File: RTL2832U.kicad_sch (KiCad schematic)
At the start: 47 parts, among them U5 RTL2832U, U6 M24C02-WMN

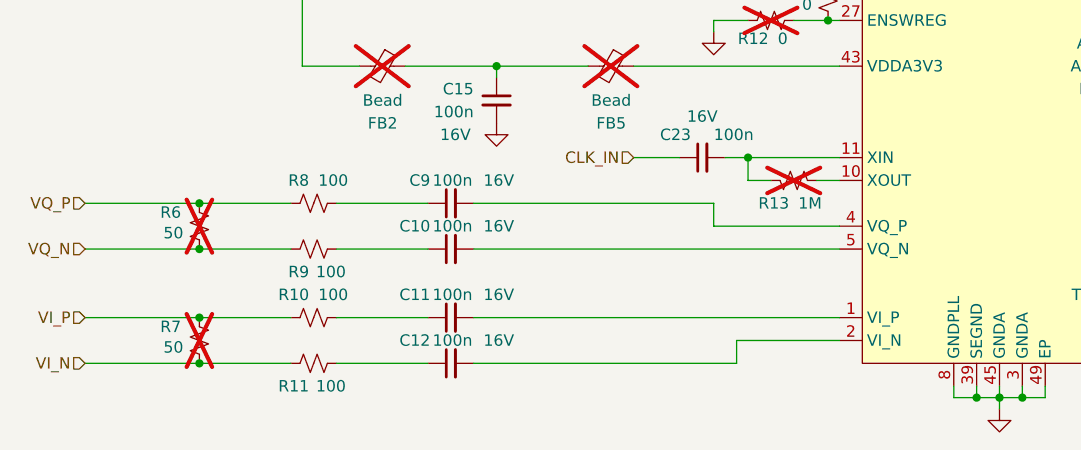
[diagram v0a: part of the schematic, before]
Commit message: PCB Layout Progress
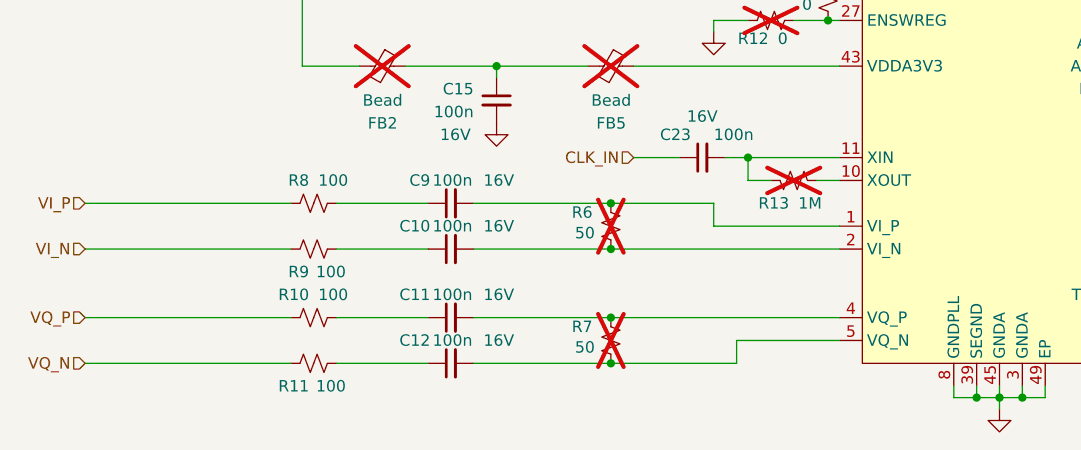
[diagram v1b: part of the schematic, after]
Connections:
- net VI_N: now also R9.2; no longer R11.2, R7.1
- net VI_P: now also R8.1; no longer R10.1, R7.2
- net VQ_N: now also R11.2; no longer R6.1, R9.2
- net VQ_P: now also R10.1; no longer R6.2, R8.1
- net at C11.2: now also R7.2, U5.4 (VQ_P); no longer U5.1 (VI_P)
- net at C10.2: now also R6.1, U5.2 (VI_N); no longer U5.5 (VQ_N)
- net at C12.2: now also R7.1, U5.5 (VQ_N); no longer U5.2 (VI_N)
- net at C9.2: now also R6.2, U5.1 (VI_P); no longer U5.4 (VQ_P)
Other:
- moved on the sheet: R6, R7
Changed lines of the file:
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@@
 	)
 	(junction
+		(at 143.51 195.58)
+		(diameter 0)
+		(color 0 0 0 0)
+	)
+	(junction
 		(at 167.64 152.4)
 		(diameter 0)
@@
 	)
 	(junction
-		(at 97.79 182.88)
-		(diameter 0)
-		(color 0 0 0 0)
-	)
-	(junction
 		(at 236.22 139.7)
 		(diameter 0)
@@
 	)
 	(junction
+		(at 143.51 182.88)
+		(diameter 0)
+		(color 0 0 0 0)
+	)
+	(junction
 		(at 184.15 204.47)
 		(diameter 0)
@@
 	)
 	(junction
+		(at 143.51 200.66)
+		(diameter 0)
+		(color 0 0 0 0)
+	)
+	(junction
 		(at 138.43 106.68)
 		(diameter 0)
@@
 	)
 	(junction
-		(at 97.79 187.96)
+		(at 231.14 144.78)
 		(diameter 0)
 		(color 0 0 0 0)
 	)
 	(junction
-		(at 231.14 144.78)
+		(at 143.51 187.96)
 		(diameter 0)
 		(color 0 0 0 0)
@@
 	)
 	(junction
-		(at 97.79 200.66)
-		(diameter 0)
-		(color 0 0 0 0)
-	)
-	(junction
 		(at 105.41 124.46)
 		(diameter 0)
@@
 	)
 	(junction
-		(at 97.79 195.58)
-		(diameter 0)
-		(color 0 0 0 0)
-	)
-	(junction
 		(at 167.64 119.38)
 		(diameter 0)
@@
 	(wire
 		(pts
-			(xy 85.09 187.96) (xy 97.79 187.96)
+			(xy 85.09 187.96) (xy 107.95 187.96)
 		)
 		(stroke
@@
 	(wire
 		(pts
-			(xy 128.27 195.58) (xy 168.91 195.58)
+			(xy 128.27 195.58) (xy 143.51 195.58)
 		)
 		(stroke
@@
 	(wire
 		(pts
+			(xy 143.51 200.66) (xy 157.48 200.66)
+		)
+		(stroke
+			(width 0)
+			(type default)
+		)
+	)
+	(wire
+		(pts
 			(xy 231.14 160.02) (xy 231.14 144.78)
 		)
@@
 	(wire
 		(pts
-			(xy 85.09 200.66) (xy 97.79 200.66)
+			(xy 85.09 200.66) (xy 107.95 200.66)
 		)
 		(stroke
@@
 	(wire
 		(pts
-			(xy 97.79 182.88) (xy 107.95 182.88)
-		)
-		(stroke
-			(width 0)
-			(type default)
-		)
-	)
-	(wire
-		(pts
-			(xy 85.09 195.58) (xy 97.79 195.58)
+			(xy 85.09 195.58) (xy 107.95 195.58)
 		)
 		(stroke
@@
 	(wire
 		(pts
-			(xy 128.27 200.66) (xy 157.48 200.66)
+			(xy 128.27 200.66) (xy 143.51 200.66)
 		)
 		(stroke
@@
 	(wire
 		(pts
+			(xy 143.51 195.58) (xy 168.91 195.58)
+		)
+		(stroke
+			(width 0)
+			(type default)
+		)
+	)
+	(wire
+		(pts
 			(xy 236.22 139.7) (xy 246.38 139.7)
 		)
@@
 	(wire
 		(pts
-			(xy 97.79 195.58) (xy 107.95 195.58)
-		)
-		(stroke
-			(width 0)
-			(type default)
-		)
-	)
-	(wire
-		(pts
 			(xy 229.87 88.9) (xy 229.87 91.44)
 		)
@@
 	(wire
 		(pts
-			(xy 85.09 182.88) (xy 97.79 182.88)
+			(xy 85.09 182.88) (xy 107.95 182.88)
+		)
+		(stroke
+			(width 0)
+			(type default)
+		)
+	)
+	(wire
+		(pts
+			(xy 143.51 182.88) (xy 154.94 182.88)
 		)
 		(stroke
@@
 	(wire
 		(pts
-			(xy 97.79 200.66) (xy 107.95 200.66)
-		)
-		(stroke
-			(width 0)
-			(type default)
-		)
-	)
-	(wire
-		(pts
 			(xy 223.52 152.4) (xy 246.38 152.4)
 		)
@@
 	(wire
 		(pts
-			(xy 97.79 187.96) (xy 107.95 187.96)
+			(xy 143.51 187.96) (xy 168.91 187.96)
 		)
 		(stroke
@@
 	(wire
 		(pts
-			(xy 128.27 187.96) (xy 168.91 187.96)
+			(xy 128.27 187.96) (xy 143.51 187.96)
 		)
 		(stroke
@@
 	(wire
 		(pts
-			(xy 128.27 182.88) (xy 154.94 182.88)
+			(xy 128.27 182.88) (xy 143.51 182.88)
 		)
 		(stroke
@@
 	(hierarchical_label "VI_N"
 		(shape input)
-		(at 85.09 200.66 180)
+		(at 85.09 187.96 180)
 		(effects
 			(font
@@
 	(hierarchical_label "VQ_P"
 		(shape input)
-		(at 85.09 182.88 180)
+		(at 85.09 195.58 180)
 		(effects
 			(font
@@
 	(hierarchical_label "VQ_N"
 		(shape input)
-		(at 85.09 187.96 180)
+		(at 85.09 200.66 180)
 		(effects
 			(font
@@
 	(hierarchical_label "VI_P"
 		(shape input)
-		(at 85.09 195.58 180)
+		(at 85.09 182.88 180)
 		(effects
 			(font
@@
 	(symbol
 		(lib_id "Device:R_Small_US")
-		(at 97.79 185.42 180)
+		(at 143.51 185.42 180)
 		(unit 1)
 		(body_style 1)
@@
 		(dnp yes)
 		(property "Reference" "R6"
-			(at 95.758 183.896 0)
+			(at 141.478 183.896 0)
 			(show_name no)
 			(do_not_autoplace no)
@@
 		)
 		(property "Value" "50"
-			(at 96.012 186.182 0)
+			(at 141.732 186.182 0)
 			(show_name no)
 			(do_not_autoplace no)
@@
 		)
 		(property "Footprint" "libraries:Worthington_R_0201"
-			(at 97.79 185.42 0)
+			(at 143.51 185.42 0)
 			(hide yes)
 			(show_name no)
@@
 		)
 		(property "Datasheet" ""
-			(at 97.79 185.42 0)
+			(at 143.51 185.42 0)
 			(hide yes)
 			(show_name no)
@@
 		)
 		(property "Description" "Resistor, small US symbol"
-			(at 97.79 185.42 0)
+			(at 143.51 185.42 0)
 			(hide yes)
 			(show_name no)
@@
 	(symbol
 		(lib_id "Device:R_Small_US")
-		(at 97.79 198.12 180)
+		(at 143.51 198.12 180)
 		(unit 1)
 		(body_style 1)
@@
 		(dnp yes)
 		(property "Reference" "R7"
-			(at 95.758 196.596 0)
+			(at 141.478 196.596 0)
 			(show_name no)
 			(do_not_autoplace no)
@@
 		)
 		(property "Value" "50"
-			(at 96.012 198.882 0)
+			(at 141.732 198.882 0)
 			(show_name no)
 			(do_not_autoplace no)
@@
 		)
 		(property "Footprint" "libraries:Worthington_R_0201"
-			(at 97.79 198.12 0)
+			(at 143.51 198.12 0)
 			(hide yes)
 			(show_name no)
@@
 		)
 		(property "Datasheet" ""
-			(at 97.79 198.12 0)
+			(at 143.51 198.12 0)
 			(hide yes)
 			(show_name no)
@@
 		)
 		(property "Description" "Resistor, small US symbol"
-			(at 97.79 198.12 0)
+			(at 143.51 198.12 0)
 			(hide yes)
 			(show_name no)

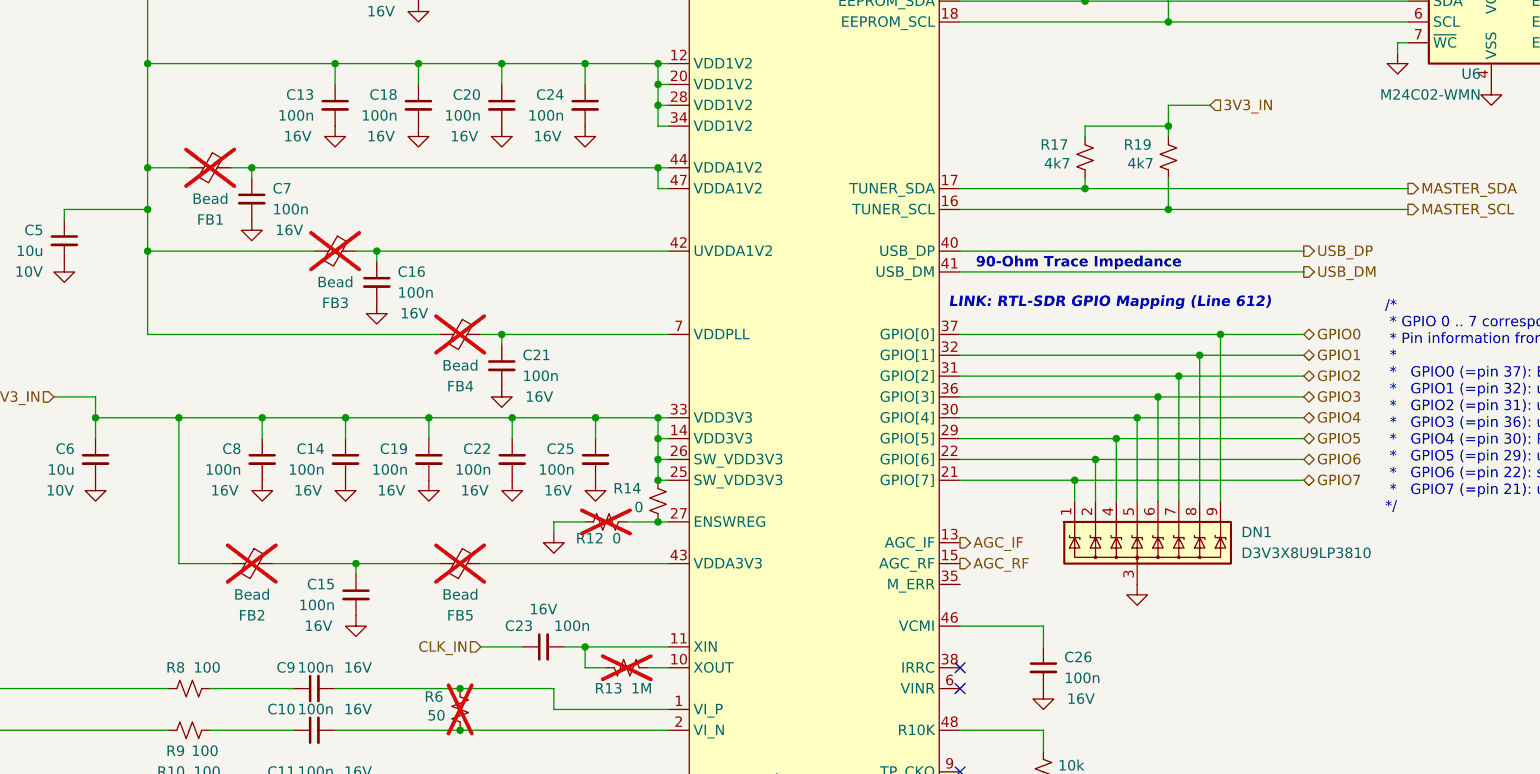
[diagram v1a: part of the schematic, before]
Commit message: PCB and schematic progress
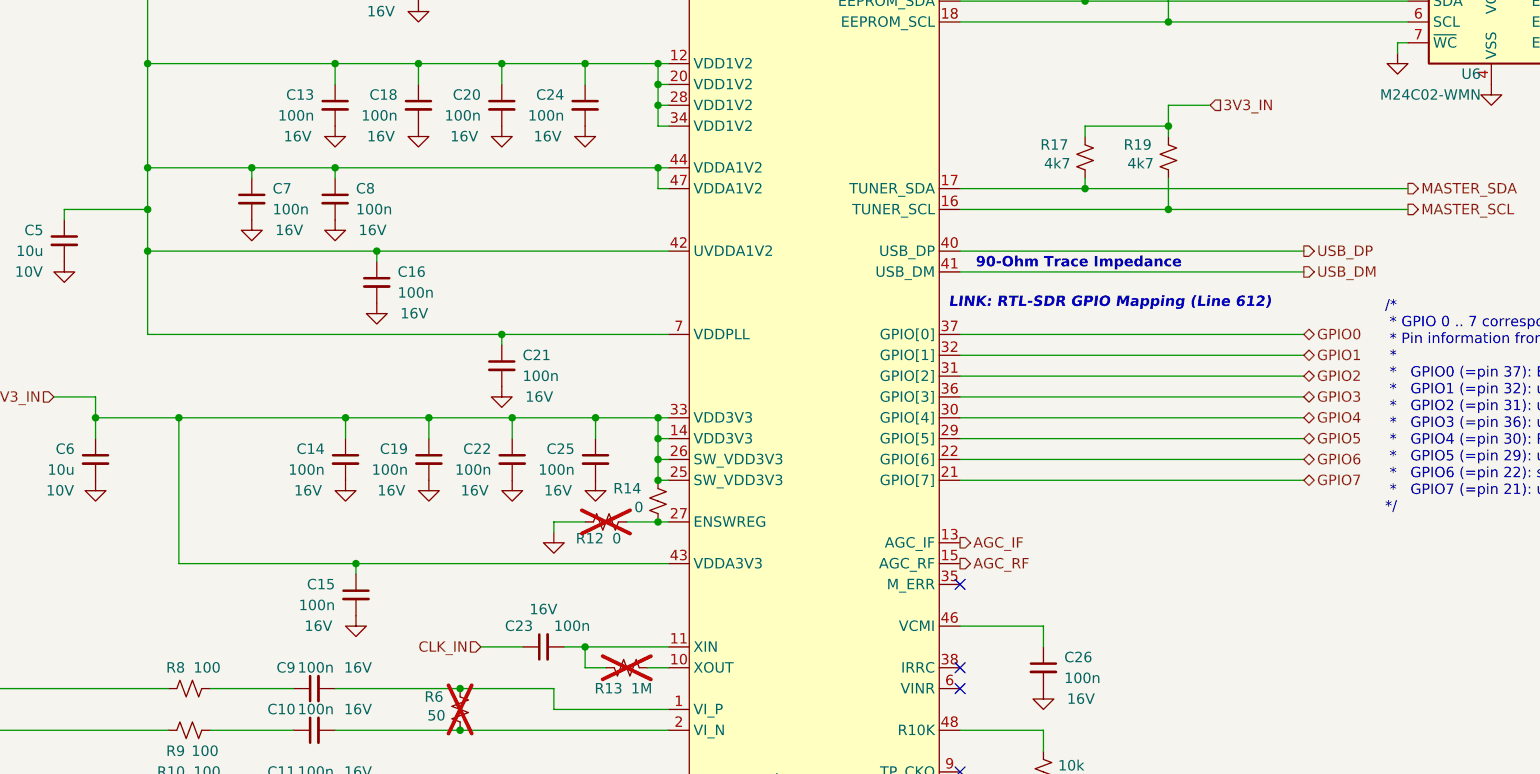
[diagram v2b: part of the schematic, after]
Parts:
- removed DN1: D3V3X8U9LP3810, Package_DFN_QFN:Diodes_UDFN3810-9_TYPE_B, symbol Power_Protection:D3V3X8U9LP3810
- removed FB1, FB2, FB3, FB4, FB5: Bead, libraries:Worthington_L_0402, symbol Device:FerriteBead_Small
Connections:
- net 3V3_IN: now also C15.1, U5.43 (VDDA3V3); no longer C8.1
- net RTL_1V2: now also C16.1, C21.1, C7.1, C8.1, U5.42 (UVDDA1V2), U5.44 (VDDA1V2), U5.47 (VDDA1V2), U5.7 (VDDPLL)
- no-connect marks 3 -> 4
